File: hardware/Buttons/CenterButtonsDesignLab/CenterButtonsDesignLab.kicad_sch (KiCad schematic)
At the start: 7 parts, among them J1 Conn_01x01, J2 Conn_01x01, J4 Conn_01x04, SW1 SW_Push, SW2 SW_Push, SW3 SW_Push, SW4 SW_Push

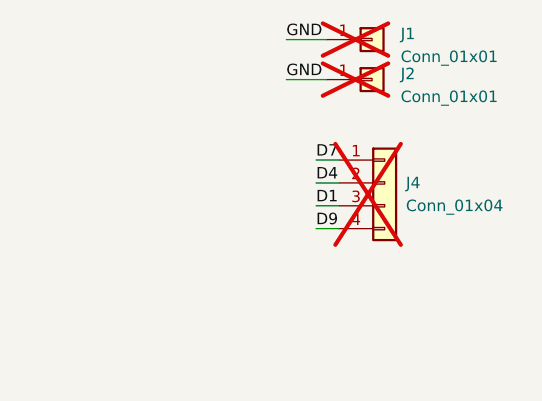
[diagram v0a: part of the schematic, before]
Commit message: Update all PCB and schematics
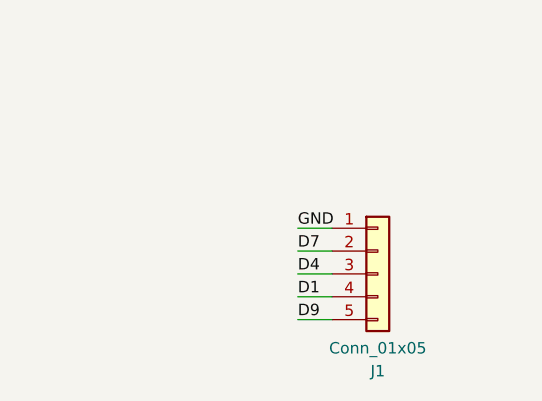
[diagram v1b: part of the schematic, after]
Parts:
- removed J1, J2: Conn_01x01, Connector_PinHeader_2.54mm:PinHeader_1x01_P2.54mm_Vertical, symbol Connector_Generic:Conn_01x01
- removed J4: Conn_01x04, Connector_PinHeader_2.54mm:PinHeader_1x04_P2.54mm_Vertical, symbol Connector_Generic:Conn_01x04
- added J1: Conn_01x05, Design:JST_S5B-PH-K-S_LF__SN_, symbol Connector_Generic:Conn_01x05
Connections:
- net D1: now also J1.4 (Pin_4)
- net D4: now also J1.3 (Pin_3)
- net D7: now also J1.2 (Pin_2)
- net D9: now also J1.5 (Pin_5)
- net GND: now also J1.1 (Pin_1)
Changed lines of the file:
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@@
     (stroke (width 0) (type default))
   )
-  (wire (pts (xy 155.575 32.385) (xy 160.02 32.385))
+  (wire (pts (xy 156.845 48.895) (xy 160.655 48.895))
     (stroke (width 0) (type default))
   )
-  (wire (pts (xy 158.877 41.3258) (xy 161.417 41.3258))
-    (stroke (width 0) (type default))
-  )
-  (wire (pts (xy 155.575 27.94) (xy 160.02 27.94))
-    (stroke (width 0) (type default))
-  )
-  (wire (pts (xy 158.877 43.8658) (xy 161.417 43.8658))
-    (stroke (width 0) (type default))
-  )
-  (wire (pts (xy 158.877 46.4058) (xy 161.417 46.4058))
-    (stroke (width 0) (type default))
-  )
-  (wire (pts (xy 158.877 48.9458) (xy 161.417 48.9458))
+  (wire (pts (xy 156.845 56.515) (xy 160.655 56.515))
     (stroke (width 0) (type default))
   )
   (wire (pts (xy 102.235 38.735) (xy 108.585 38.735))
+    (stroke (width 0) (type default))
+  )
+  (wire (pts (xy 156.845 51.435) (xy 160.655 51.435))
+    (stroke (width 0) (type default))
+  )
+  (wire (pts (xy 156.845 59.055) (xy 160.655 59.055))
     (stroke (width 0) (type default))
   )
@@
     (stroke (width 0) (type default))
   )
+  (wire (pts (xy 156.845 53.975) (xy 160.655 53.975))
+    (stroke (width 0) (type default))
+  )
   (label "D9" (at 84.6328 58.2168 0) (fields_autoplaced)
     (effects (font (size 1.27 1.27)) (justify left bottom))
   )
-  (label "D1" (at 158.877 46.4058 0) (fields_autoplaced)
+  (label "GND" (at 156.845 48.895 0) (fields_autoplaced)
     (effects (font (size 1.27 1.27)) (justify left bottom))
   )
-  (label "D4" (at 158.877 43.8658 0) (fields_autoplaced)
+  (label "D1" (at 156.845 56.515 0) (fields_autoplaced)
+    (effects (font (size 1.27 1.27)) (justify left bottom))
+  )
+  (label "D4" (at 156.845 53.975 0) (fields_autoplaced)
     (effects (font (size 1.27 1.27)) (justify left bottom))
   )
@@
     (effects (font (size 1.27 1.27)) (justify left bottom))
   )
-  (label "GND" (at 155.575 32.385 0) (fields_autoplaced)
-    (effects (font (size 1.27 1.27)) (justify left bottom))
-  )
-  (label "D7" (at 158.877 41.3258 0) (fields_autoplaced)
+  (label "D7" (at 156.845 51.435 0) (fields_autoplaced)
     (effects (font (size 1.27 1.27)) (justify left bottom))
   )
@@
     (effects (font (size 1.27 1.27)) (justify left bottom))
   )
-  (label "D9" (at 158.877 48.9458 0) (fields_autoplaced)
+  (label "D9" (at 156.845 59.055 0) (fields_autoplaced)
     (effects (font (size 1.27 1.27)) (justify left bottom))
   )
@@
     (effects (font (size 1.27 1.27)) (justify left bottom))
   )
-  (label "GND" (at 155.575 27.94 0) (fields_autoplaced)
-    (effects (font (size 1.27 1.27)) (justify left bottom))
+  (symbol (lib_id "Connector_Generic:Conn_01x05") (at 165.735 53.975 0) (unit 1)
+    (in_bom yes) (on_board yes) (dnp no)
+    (property "Reference" "J1" (at 165.735 64.77 0)
+      (effects (font (size 1.27 1.27)))
+    )
+    (property "Value" "Conn_01x05" (at 165.735 62.23 0)
+      (effects (font (size 1.27 1.27)))
+    )
+    (property "Footprint" "Design:JST_S5B-PH-K-S_LF__SN_" (at 165.735 53.975 0)
+      (effects (font (size 1.27 1.27)) hide)
+    )
+    (property "Datasheet" "https://datasheet.lcsc.com/lcsc/2304140030_JST-S5B-PH-K-S-LF-SN_C157923.pdf" (at 165.735 53.975 0)
+      (effects (font (size 1.27 1.27)) hide)
+    )
+    (property "LCSC#" "C157923" (at 165.735 53.975 0)
+      (effects (font (size 1.27 1.27)) hide)
+    )
+    (pin "1")
+    (pin "2")
+    (pin "3")
+    (pin "4")
+    (pin "5")
+    (instances
+      (project "CenterButtonsDesignLab"
+        (path "/60a80ef2-fa88-492e-9ae7-a70a1d03dbe3"
+          (reference "J1") (unit 1)
+        )
+      )
+    )
   )
   (symbol (lib_id "Switch:SW_Push") (at 76.835 38.735 0) (unit 1)
@@
         )
       )
-    )
-  )
-  (symbol (lib_id "Connector_Generic:Conn_01x01") (at 165.1 32.385 0) (unit 1)
-    (in_bom yes) (on_board yes) (dnp yes) (fields_autoplaced)
-    (property "Reference" "J2" (at 168.275 31.75 0)
-      (effects (font (size 1.27 1.27)) (justify left))
-    )
-    (property "Value" "Conn_01x01" (at 168.275 34.29 0)
-      (effects (font (size 1.27 1.27)) (justify left))
-    )
-    (property "Footprint" "Connector_PinHeader_2.54mm:PinHeader_1x01_P2.54mm_Vertical" (at 165.1 32.385 0)
-      (effects (font (size 1.27 1.27)) hide)
-    )
-    (property "Datasheet" "~" (at 165.1 32.385 0)
-      (effects (font (size 1.27 1.27)) hide)
-    )
-    (pin "1")
-    (instances
-      (project "CenterButtonsDesignLab"
-        (path "/60a80ef2-fa88-492e-9ae7-a70a1d03dbe3"
-          (reference "J2") (unit 1)
-        )
-      )
-      (project "ButtonDesignLab"
-        (path "/e63e39d7-6ac0-4ffd-8aa3-1841a4541b55"
-          (reference "J4") (unit 1)
-        )
-      )
-    )
-  )
-  (symbol (lib_id "Connector_Generic:Conn_01x04") (at 166.497 43.8658 0) (unit 1)
-    (in_bom yes) (on_board yes) (dnp yes) (fields_autoplaced)
-    (property "Reference" "J4" (at 168.8592 43.8658 0)
-      (effects (font (size 1.27 1.27)) (justify left))
-    )
-    (property "Value" "Conn_01x04" (at 168.8592 46.4058 0)
-      (effects (font (size 1.27 1.27)) (justify left))
-    )
-    (property "Footprint" "Connector_PinHeader_2.54mm:PinHeader_1x04_P2.54mm_Vertical" (at 166.497 43.8658 0)
-      (effects (font (size 1.27 1.27)) hide)
-    )
-    (property "Datasheet" "~" (at 166.497 43.8658 0)
-      (effects (font (size 1.27 1.27)) hide)
-    )
-    (pin "1")
-    (pin "2")
-    (pin "3")
-    (pin "4")
-    (instances
-      (project "CenterButtonsDesignLab"
-        (path "/60a80ef2-fa88-492e-9ae7-a70a1d03dbe3"
-          (reference "J4") (unit 1)
-        )
-      )
-    )
-  )
-  (symbol (lib_id "Connector_Generic:Conn_01x01") (at 165.1 27.94 0) (unit 1)
-    (in_bom yes) (on_board yes) (dnp yes) (fields_autoplaced)
-    (property "Reference" "J1" (at 168.275 27.305 0)
-      (effects (font (size 1.27 1.27)) (justify left))
-    )
-    (property "Value" "Conn_01x01" (at 168.275 29.845 0)
-      (effects (font (size 1.27 1.27)) (justify left))
-    )
-    (property "Footprint" "Connector_PinHeader_2.54mm:PinHeader_1x01_P2.54mm_Vertical" (at 165.1 27.94 0)
-      (effects (font (size 1.27 1.27)) hide)
-    )
-    (property "Datasheet" "~" (at 165.1 27.94 0)
-      (effects (font (size 1.27 1.27)) hide)
-    )
-    (pin "1")
-    (instances
-      (project "CenterButtonsDesignLab"
-        (path "/60a80ef2-fa88-492e-9ae7-a70a1d03dbe3"
-          (reference "J1") (unit 1)
-        )
-      )
-      (project "ButtonDesignLab"
-        (path "/e63e39d7-6ac0-4ffd-8aa3-1841a4541b55"
-          (reference "J5") (unit 1)
-        )
-      )

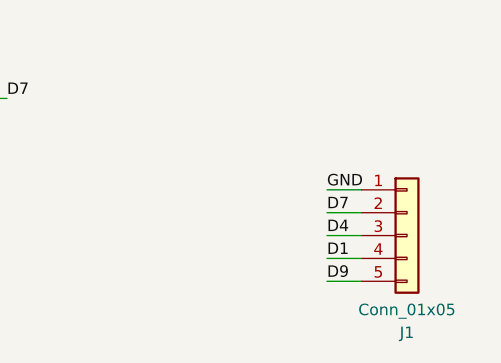
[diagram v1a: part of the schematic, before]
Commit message: Update PCB
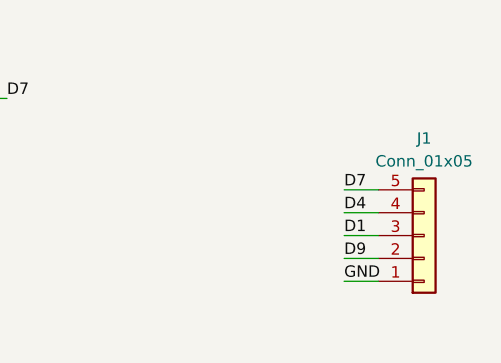
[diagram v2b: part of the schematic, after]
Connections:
- net D1: now also J1.3 (Pin_3); no longer J1.4 (Pin_4)
- net D4: now also J1.4 (Pin_4); no longer J1.3 (Pin_3)
- net D7: now also J1.5 (Pin_5); no longer J1.2 (Pin_2)
- net D9: now also J1.2 (Pin_2); no longer J1.5 (Pin_5)
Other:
- moved on the sheet: J1
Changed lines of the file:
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@@
     (stroke (width 0) (type default))
   )
-  (wire (pts (xy 156.845 48.895) (xy 160.655 48.895))
+  (wire (pts (xy 158.75 59.055) (xy 162.56 59.055))
     (stroke (width 0) (type default))
   )
-  (wire (pts (xy 156.845 56.515) (xy 160.655 56.515))
+  (wire (pts (xy 158.75 53.975) (xy 162.56 53.975))
     (stroke (width 0) (type default))
   )
@@
     (stroke (width 0) (type default))
   )
-  (wire (pts (xy 156.845 51.435) (xy 160.655 51.435))
+  (wire (pts (xy 158.75 48.895) (xy 162.56 48.895))
     (stroke (width 0) (type default))
   )
-  (wire (pts (xy 156.845 59.055) (xy 160.655 59.055))
+  (wire (pts (xy 158.75 56.515) (xy 162.56 56.515))
     (stroke (width 0) (type default))
   )
@@
     (stroke (width 0) (type default))
   )
-  (wire (pts (xy 156.845 53.975) (xy 160.655 53.975))
+  (wire (pts (xy 158.75 51.435) (xy 162.56 51.435))
     (stroke (width 0) (type default))
   )
@@
     (effects (font (size 1.27 1.27)) (justify left bottom))
   )
-  (label "GND" (at 156.845 48.895 0) (fields_autoplaced)
+  (label "GND" (at 158.75 59.055 0) (fields_autoplaced)
     (effects (font (size 1.27 1.27)) (justify left bottom))
   )
-  (label "D1" (at 156.845 56.515 0) (fields_autoplaced)
+  (label "D1" (at 158.75 53.975 0) (fields_autoplaced)
     (effects (font (size 1.27 1.27)) (justify left bottom))
   )
-  (label "D4" (at 156.845 53.975 0) (fields_autoplaced)
+  (label "D4" (at 158.75 51.435 0) (fields_autoplaced)
     (effects (font (size 1.27 1.27)) (justify left bottom))
   )
@@
     (effects (font (size 1.27 1.27)) (justify left bottom))
   )
-  (label "D7" (at 156.845 51.435 0) (fields_autoplaced)
+  (label "D7" (at 158.75 48.895 0) (fields_autoplaced)
     (effects (font (size 1.27 1.27)) (justify left bottom))
   )
@@
     (effects (font (size 1.27 1.27)) (justify left bottom))
   )
-  (label "D9" (at 156.845 59.055 0) (fields_autoplaced)
+  (label "D9" (at 158.75 56.515 0) (fields_autoplaced)
     (effects (font (size 1.27 1.27)) (justify left bottom))
   )
@@
     (effects (font (size 1.27 1.27)) (justify left bottom))
   )
-  (symbol (lib_id "Connector_Generic:Conn_01x05") (at 165.735 53.975 0) (unit 1)
+  (symbol (lib_id "Connector_Generic:Conn_01x05") (at 167.64 53.975 0) (mirror x) (unit 1)
     (in_bom yes) (on_board yes) (dnp no)
-    (property "Reference" "J1" (at 165.735 64.77 0)
+    (property "Reference" "J1" (at 167.64 43.18 0)
       (effects (font (size 1.27 1.27)))
     )
-    (property "Value" "Conn_01x05" (at 165.735 62.23 0)
+    (property "Value" "Conn_01x05" (at 167.64 45.72 0)
       (effects (font (size 1.27 1.27)))
     )
-    (property "Footprint" "Design:JST_S5B-PH-K-S_LF__SN_" (at 165.735 53.975 0)
+    (property "Footprint" "Design:JST_S5B-PH-K-S_LF__SN_" (at 167.64 53.975 0)
       (effects (font (size 1.27 1.27)) hide)
     )
-    (property "Datasheet" "https://datasheet.lcsc.com/lcsc/2304140030_JST-S5B-PH-K-S-LF-SN_C157923.pdf" (at 165.735 53.975 0)
+    (property "Datasheet" "https://datasheet.lcsc.com/lcsc/2304140030_JST-S5B-PH-K-S-LF-SN_C157923.pdf" (at 167.64 53.975 0)
       (effects (font (size 1.27 1.27)) hide)
     )
-    (property "LCSC#" "C157923" (at 165.735 53.975 0)
+    (property "LCSC#" "C157923" (at 167.64 53.975 0)
       (effects (font (size 1.27 1.27)) hide)
     )
